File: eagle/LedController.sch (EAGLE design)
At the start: 31 parts, among them IC1 MCP601R, Q2 FA-238, Q5 PMV20EN, X2 MKDSN1,5/4-5,08

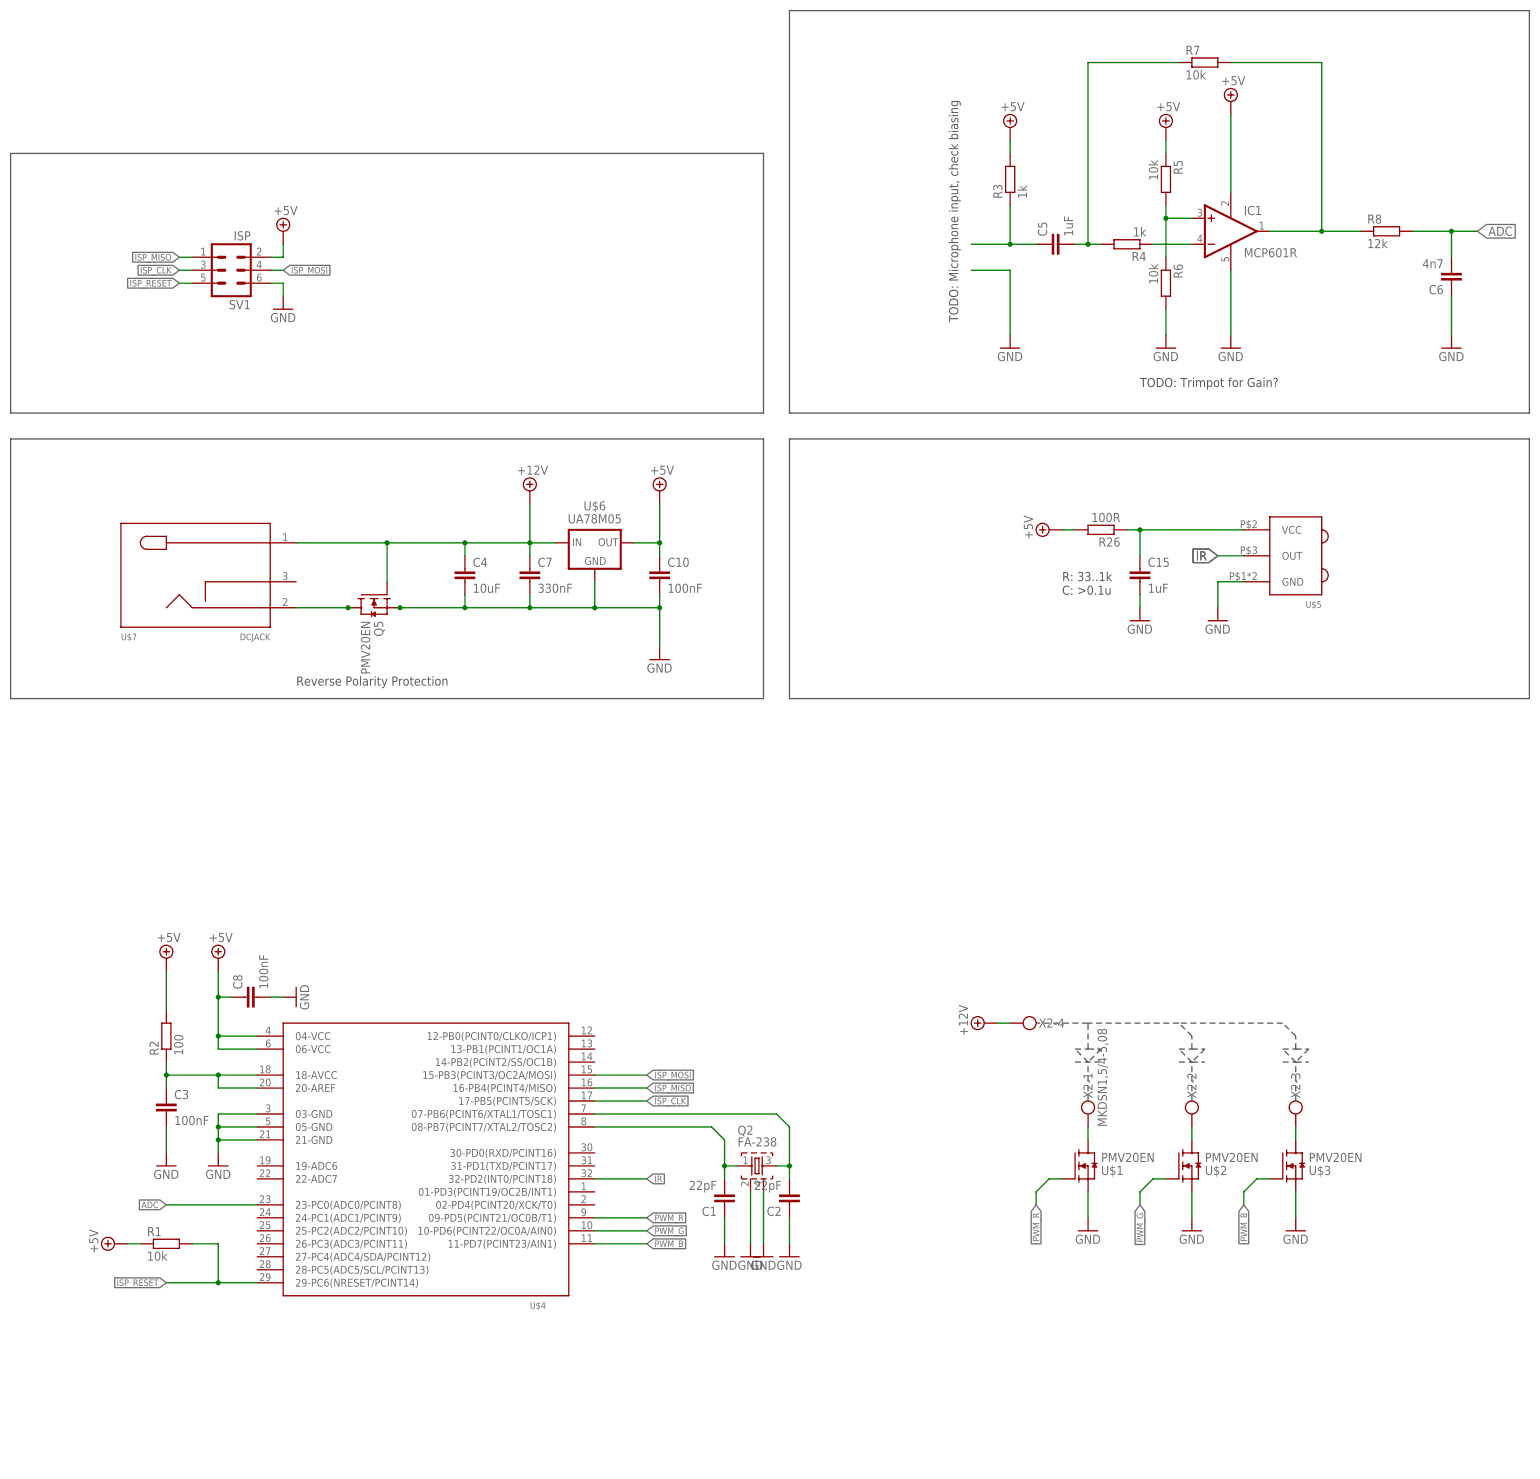
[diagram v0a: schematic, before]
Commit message: More relayouting, Framed schematic
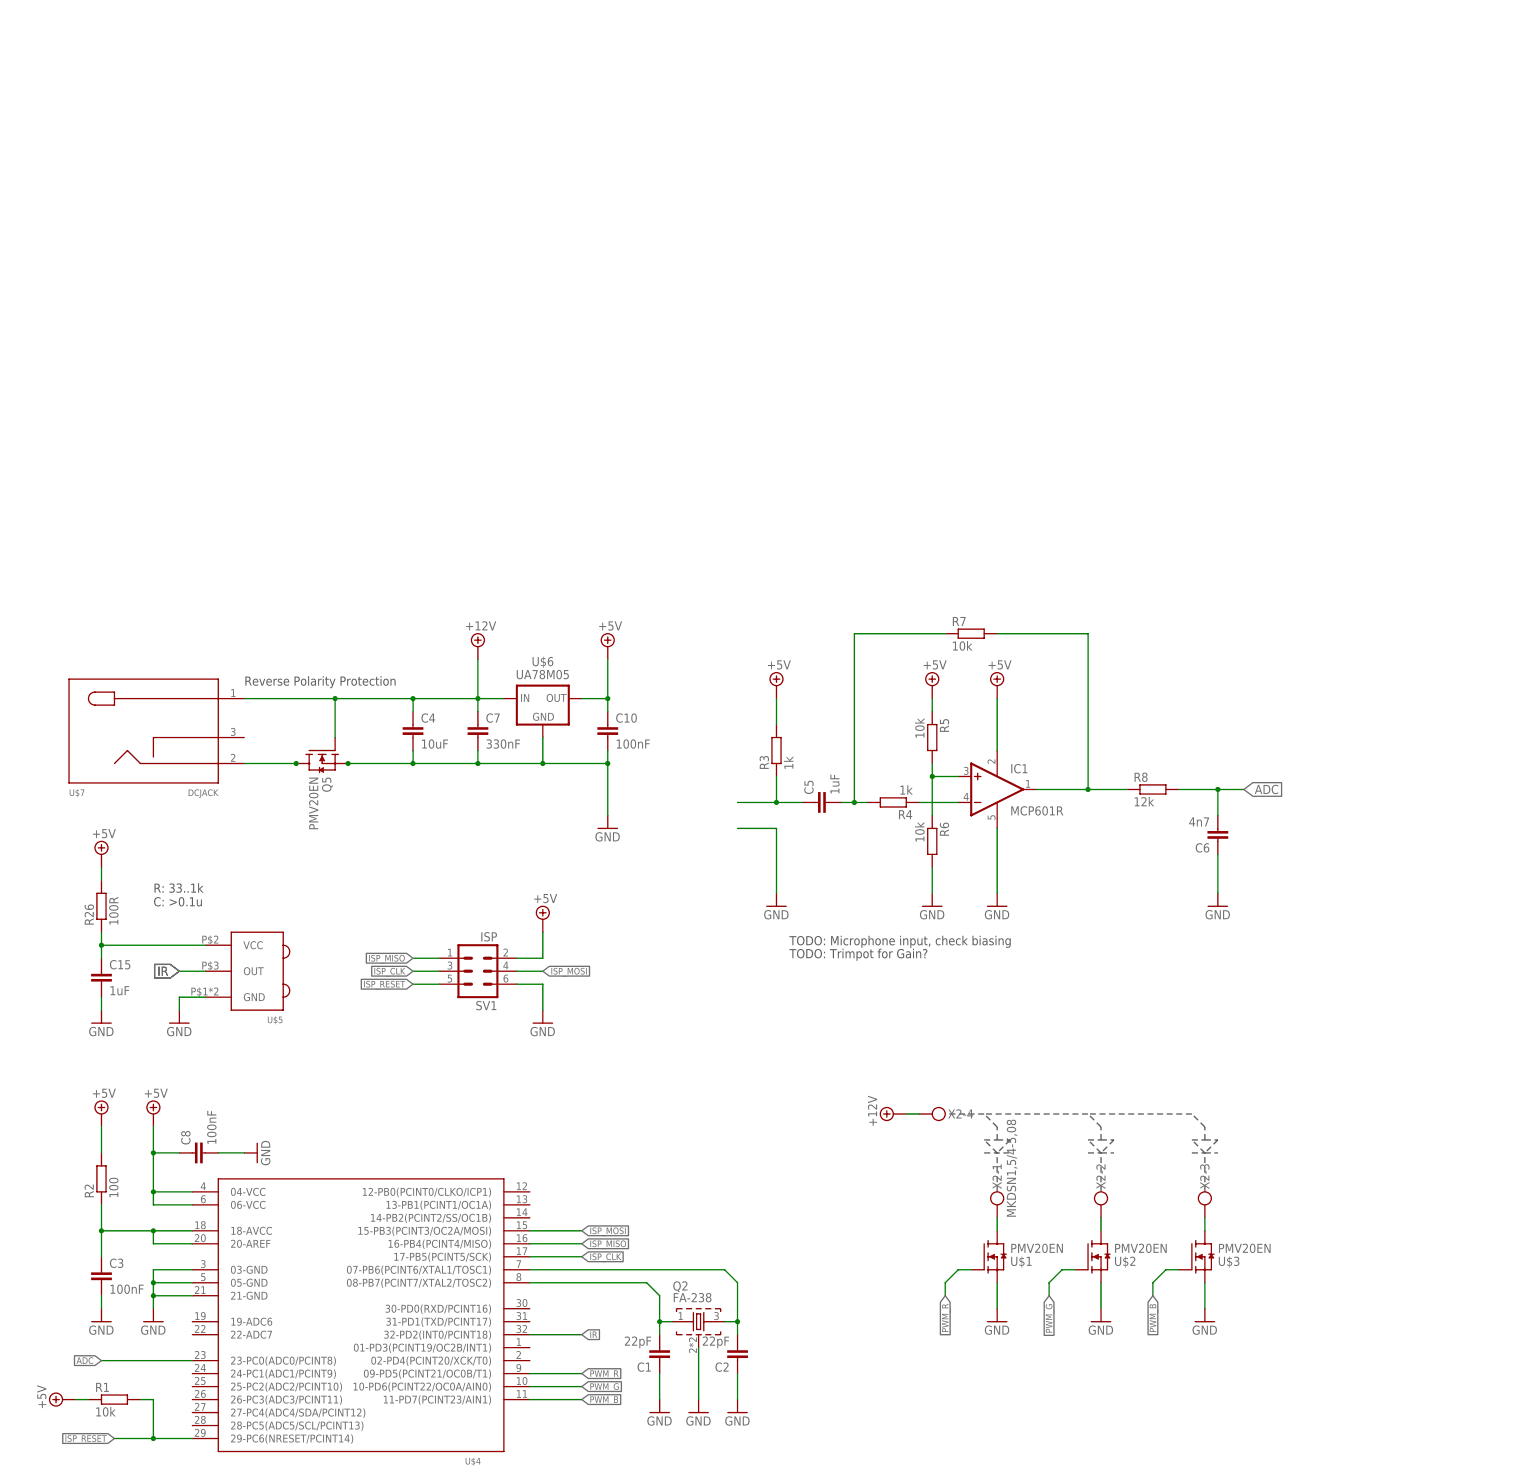
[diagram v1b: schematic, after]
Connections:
- net GND: no longer Q2.4
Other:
- moved on the sheet: C1, C10, C15, C2, C3, C4, C5, C6, C7, C8, IC1, Q5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
